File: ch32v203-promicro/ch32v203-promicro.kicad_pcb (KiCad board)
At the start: 2 copper layers, 17.8 x 33 mm, 30 parts, among them J1 USB2.0_C_v3, J2 ProMicro-LeftPin-NoGND, J3 ProMicro-RightPin, SW1 SW_Push, SW2 SW_Push, U1 STM32V103C8T6, U2 AMS1117-3.3, Y1 32.768k, Y2 8M

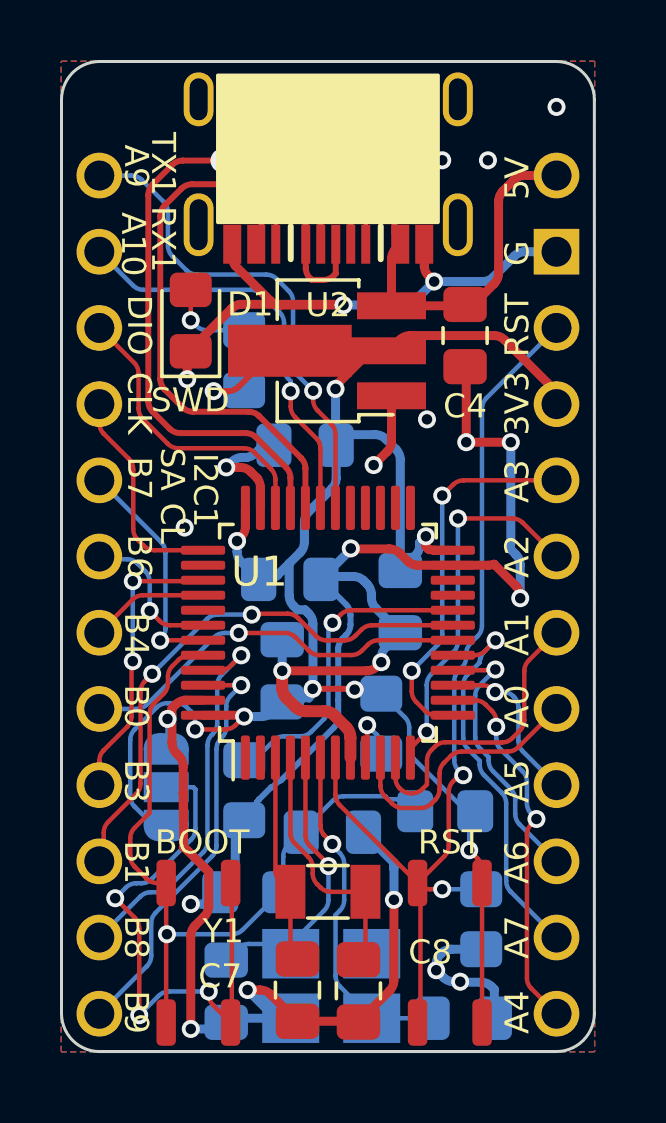
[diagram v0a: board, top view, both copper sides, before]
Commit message: v1.2.0
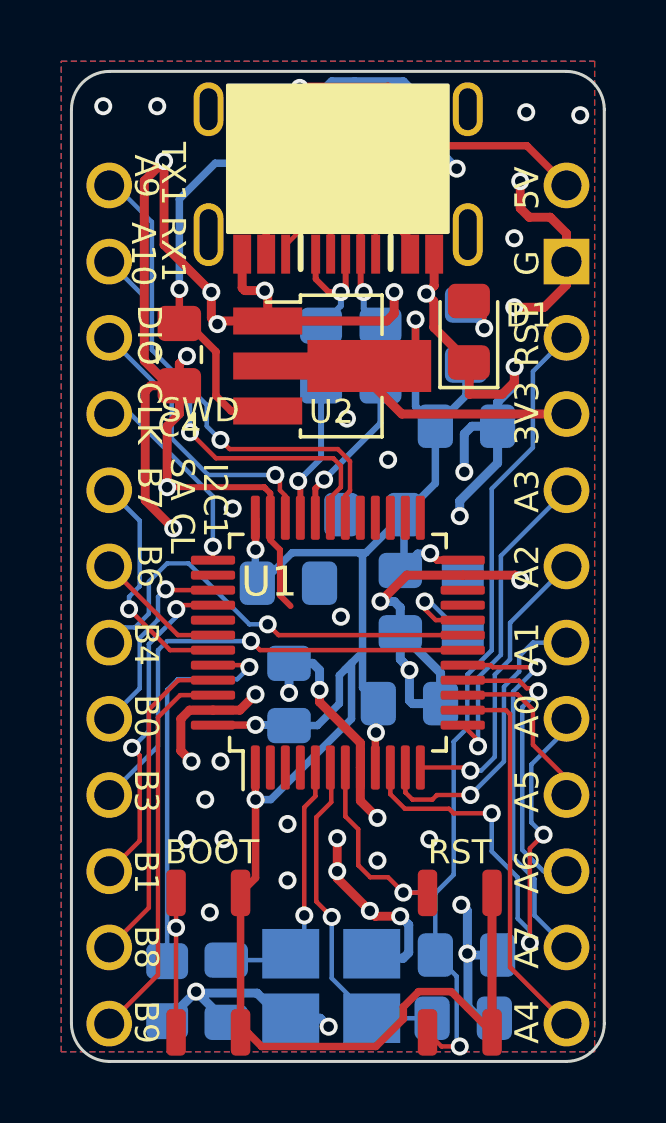
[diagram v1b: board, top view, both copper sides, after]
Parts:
- removed C8: 12p, $74th:Capacitor_0805_2012
- removed J2: ProMicro-LeftPin-NoGND, $74th:ProMicro_LIKE_LEFT_NO_GND
- removed J3: ProMicro-RightPin, $74th:ProMicro_LIKE_RIGHT
- removed JP1: Jumper_3_Open, Jumper:SolderJumper-3_P1.3mm_Open_RoundedPad1.0x1.5mm
- removed R3: 0, $74th:Register_0805_2012
- removed R6: 10k, $74th:Register_0805_2012
- removed Y1: 32.768k, $74th:Crystal_SMD_3215-2Pin_3.2x1.5mm
- added C11: 1u, $74th:Capacitor_0805_2012, B.Cu at (110.4, 115.1)
- added J5: ProMicro-LeftPin-NoGND, $74th:ProMicro_LIKE_LEFT_NO_GND, F.Cu at (101.6, 118.1)
- added J6: ProMicro-RightPin, $74th:ProMicro_LIKE_RIGHT, F.Cu at (116.8, 119.4)
- added R9: 27.4, $74th:Register_0805_2012, B.Cu at (108.7, 109.8)
- added U4: CH213K, Package_TO_SOT_SMD:SOT-23, B.Cu at (107.1, 102.5)
- C5: value 2.2u -> 10u
- C7: value 12p -> 100n; moved to B.Cu
- D1: value LED -> BLUE
- R1: value 200 -> 10k
- R2: value 10k -> 27.4
- moved R2 15.2 mm to (110.6, 109.8), turned to -90 degrees
- moved C7 13.6 mm to (107.6, 117.4), turned to 0 degrees
- moved R7 9.70 mm to (113.4, 118.1), turned to 90 degrees
- moved C4 9.55 mm to (103.9, 109.8)
- moved D1 9.28 mm to (113.6, 109.0)
- moved R1 7.44 mm to (113.6, 109.0)
- moved C6 6.06 mm to (113.5, 129.8)
- moved C2 5.75 mm to (111.6, 121.4)
- moved C5 5.42 mm to (113.5, 112.2), turned to 0 degrees
- moved R8 4.32 mm to (103.5, 131.0), turned to -90 degrees
- moved R4 1.99 mm to (109.9, 103.0)
- moved R5 1.90 mm to (111.8, 103.0)
- moved C3 0.82 mm to (107.6, 121.1)
- moved U2 0.54 mm to (109.0, 110.2), turned to 0 degrees
- moved SW1 0.47 mm to (113.3, 130.0)
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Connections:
- net BOOT1 renamed Net-(U1-BOOT1/PB2)
- C4 pad 1: +5V -> Net-(U2-VI)
- C6 pad 1: BOOT0 -> /~{RESET}
- C7 pad 1: Net-(U1-PC14/OSC32IN) -> +3V3
- J1 pad 2: DM -> Net-(J1-D-)
- J1 pad 3: DP -> Net-(J1-D+)
- R2 pad 1: +3V3 -> Net-(J1-D-)
- R2 pad 2: BOOT0 -> /USB_DM
- R8 pad 1: BOOT0 -> Net-(U1-BOOT0)
- SW1 pad 2: RST -> /~{RESET}
- SW2 pad 1: Net-(JP1-C) -> +3V3
- SW2 pad 2: BOOT0 -> Net-(U1-BOOT0)
- U1 pad 1: unconnected-(U1-VBAT-Pad1) -> +3V3
- U1 pad 10: 18/A0 -> /18/A0
- U1 pad 11: 19/A1 -> /19/A1
- U1 pad 12: 20/A2 -> /20/A2
- U1 pad 13: 21/A3 -> /21/A3
- U1 pad 14: 10/A10 -> /10/A10
- U1 pad 15: 15/SPI_SCK -> /15/SPI_SCK
- U1 pad 16: 14/SPI_MISO -> /14/SPI_MISO
- U1 pad 17: 16/SPI_MOSI -> /16/SPI_MOSI
- U1 pad 18: 5 -> /6/A7
- U1 pad 19: 7 -> /4/A6
- U1 pad 3: Net-(U1-PC14/OSC32IN) -> unconnected-(U1-PC14/OSC32IN-Pad3)
- U1 pad 30: 1/UART_TX -> /1/UART_TX
- U1 pad 31: 0/UART_RX -> /0/UART_RX
- U1 pad 32: DM -> /USB_DM
- U1 pad 33: DP -> /USB_DP
- U1 pad 34: SWDIO -> /SWDIO
- U1 pad 37: SWCLK -> /SWCLK
- U1 pad 39: 6/A7 -> /5
- U1 pad 4: Net-(U1-PC15/OSC32OUT) -> unconnected-(U1-PC15/OSC32OUT-Pad4)
- U1 pad 40: 4/A6 -> /7
- U1 pad 42: 3/I2C_SCL -> /3/ISC_SCL
- U1 pad 43: 2/I2C_SDA -> /2/ISC_SDA
- U1 pad 44: BOOT0 -> Net-(U1-BOOT0)
- U1 pad 45: 8/A8 -> /8/A8
- U1 pad 46: 9/A9 -> /9/A9
- U1 pad 7: RST -> /~{RESET}
- U1 pad 9: Net-(U1-VDDA) -> +3V3
- U2 pad 3: +5V -> Net-(U2-VI)
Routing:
- net /~{RESET}: track 0.00 -> 34.2 mm, vias 0 -> 2
- net RST: track 32.8 -> 0.00 mm, vias 2 -> 0
- net DM: track 28.5 -> 0.00 mm, vias 2 -> 0
- net BOOT0: track 25.0 -> 0.00 mm, vias 1 -> 0
- net DP: track 24.4 -> 0.00 mm, vias 2 -> 0
- net Net-(JP1-C): track 18.8 -> 0.00 mm, vias 3 -> 0
- net GND: track 110.5 -> 129.1 mm, vias 23 -> 53
- net Net-(U1-BOOT0): track 0.00 -> 18.3 mm, vias 0 -> 2
- net 7: track 18.2 -> 0.00 mm, vias 2 -> 0
- net /18/A0: track 0.00 -> 17.3 mm, vias 0 -> 3
- net /1/UART_TX: track 0.00 -> 16.5 mm, vias 0 -> 1
- net 1/UART_TX: track 16.5 -> 0.00 mm, vias 1 -> 0
- net /6/A7: track 0.00 -> 15.9 mm, vias 0 -> 1
- net /4/A6: track 0.00 -> 14.5 mm, vias 0 -> 1
- net /0/UART_RX: track 0.00 -> 14.2 mm, vias 0 -> 1
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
